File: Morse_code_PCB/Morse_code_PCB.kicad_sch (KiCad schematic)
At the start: 14 parts, among them J1 USB_C_Receptacle_USB2.0, J2 AudioJack3_Ground, J3 AudioJack3_Ground, SW1 RotaryEncoder_Switch, U1 STM32F030F4Px, U2 OLED_12864

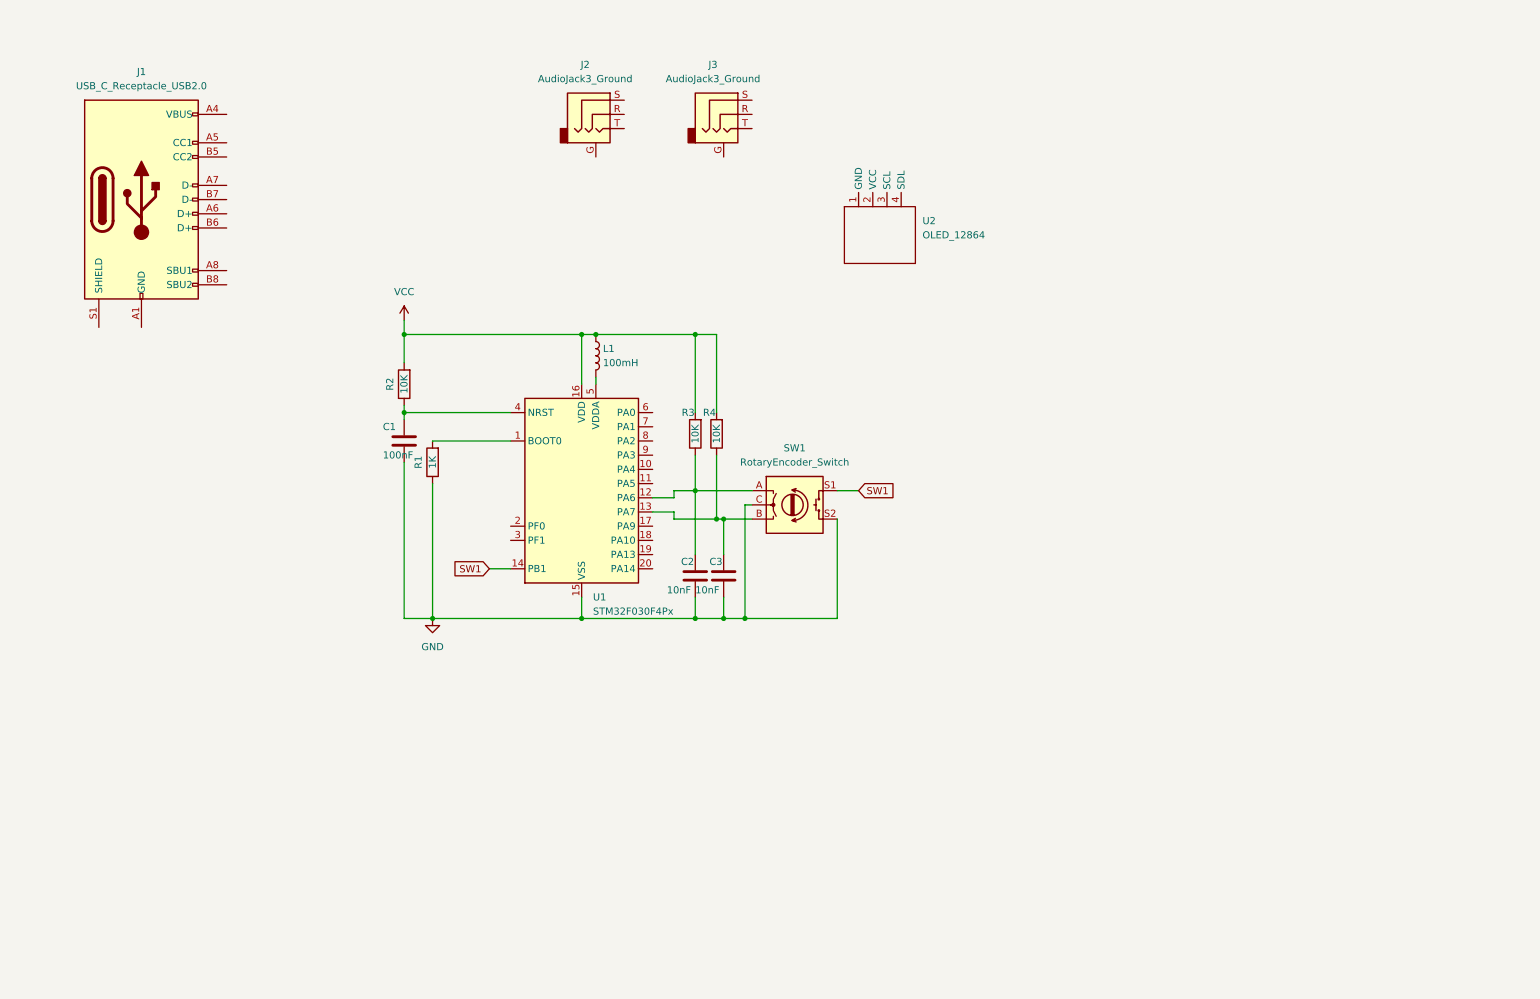
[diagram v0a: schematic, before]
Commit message: 摸鱼画了一点 Signed-off-by: kevin <kevin@lmve.net>
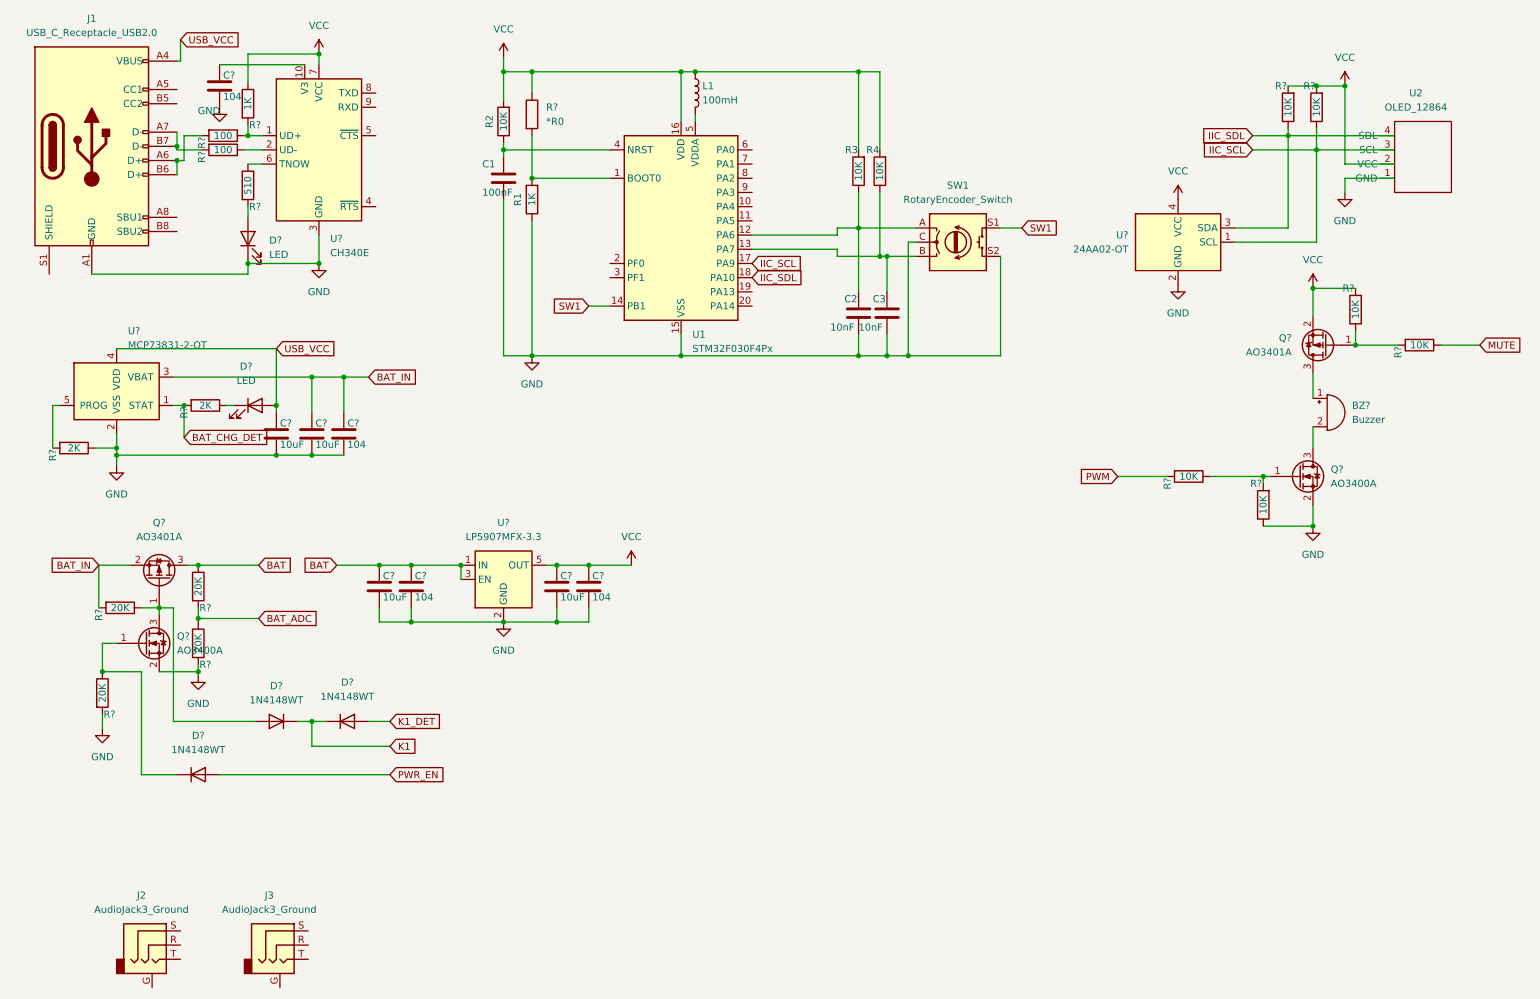
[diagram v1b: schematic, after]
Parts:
- added BZ?: Buzzer, Buzzer_Beeper:Buzzer_TDK_PS1240P02BT_D12.2mm_H6.5mm, symbol Device:Buzzer
- added C? (x4): 10uF, Capacitor_SMD:C_2220_5650Metric, symbol Device:C
- added C? (x4): 104, Capacitor_SMD:C_0805_2012Metric, symbol Device:C
- added D? (x3): 1N4148WT, Diode_SMD:D_SOD-523, symbol Diode:1N4148WT
- added D? (x2): LED, LED_SMD:LED_0603_1608Metric, symbol Device:LED
- added Q? (x2): AO3401A, Package_TO_SOT_SMD:SOT-23, symbol Transistor_FET:AO3401A
- added Q? (x2): AO3400A, Package_TO_SOT_SMD:SOT-23, symbol Transistor_FET:AO3400A
- added R? (x2): 100, Resistor_SMD:R_0603_1608Metric, symbol Device:R
- added R? (x6): 10K, Resistor_SMD:R_0603_1608Metric, symbol Device:R
- added R? (x4): 20K, Resistor_SMD:R_0603_1608Metric, symbol Device:R
- added R?: 510, Resistor_SMD:R_0603_1608Metric, symbol Device:R
- added R? (x2): 2K, Resistor_SMD:R_0603_1608Metric, symbol Device:R
- added R?: 1K, Resistor_SMD:R_0603_1608Metric, symbol Device:R
- added R?: *R0, Resistor_SMD:R_0402_1005Metric, symbol Device:R
- added U?: MCP73831-2-OT, Package_TO_SOT_SMD:SOT-23-5, symbol Battery_Management:MCP73831-2-OT
- added U?: 24AA02-OT, Package_SO:TSSOP-8_4.4x3mm_P0.65mm, symbol Memory_EEPROM:24AA02-OT
- added U?: CH340E, Package_SO:MSOP-10_3x3mm_P0.5mm, symbol Interface_USB:CH340E
- added U?: LP5907MFX-3.3, Package_TO_SOT_SMD:SOT-23-5, symbol Regulator_Linear:LP5907MFX-3.3
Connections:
- net GND: now also J1.A1 (GND), J1.A12 (GND), J1.B1 (GND), J1.B12 (GND), U2.1 (GND), C?.2, C?.2, C?.2, C?.2, C?.2, C?.2, C?.2, C?.2, D?.1 (K), Q?.2 (S), Q?.2 (S), R?.1, R?.1, R?.2, R?.2, U?.2 (GND), U?.2 (GND), U?.2 (VSS), U?.3 (GND)
- net VCC: now also U2.2 (VCC), C?.1, C?.1, Q?.2 (S), R?.1, R?.1, R?.2, R?.2, R?.2, U?.4 (VCC), U?.5 (OUT), U?.7 (VCC)
- net IIC_SCL: now reaches U2.3 (SCL)
- net IIC_SCL: now also U1.17 (PA9), R?.1, U?.1 (SCL)
- net IIC_SDL: now reaches U2.4 (SDL)
- net IIC_SDL: now also U1.18 (PA10), R?.1, U?.3 (SDA)
- net at R1.2, U1.1 (BOOT0): now also R?.2
- net USB_VCC: now reaches J1.A4 (VBUS), J1.A9 (VBUS), J1.B4 (VBUS), J1.B9 (VBUS)
- net USB_VCC: now also C?.1, D?.2 (A), U?.4 (VDD)
- net at J1.A6 (D+): now also J1.B6 (D+), R?.2
- net at J1.A7 (D-): now also J1.B7 (D-), R?.2
- new net: R?.1, R?.2, U?.1 (UD+)
- new net: Q?.1 (G), R?.1, R?.2 (x2)
- new net: D?.2 (A), Q?.1 (G), Q?.3 (D), R?.1
- new net: D?.1 (K), Q?.1 (G), R?.1
- new net: R?.1, U?.2 (UD-)
- new net: R?.1, U?.6 (TNOW)
- new net: D?.2 (A), R?.2
- new net: C?.1, U?.10 (V3)
- new net: BZ?.1 (-), Q?.3 (D)
- new net: BZ?.2 (+), Q?.3 (D)
- new net: D?.1 (K), R?.1
- new net: R?.2, U?.5 (PROG)
- new net BAT: C?.1, C?.1, Q?.3 (D), R?.1, U?.1 (IN), U?.3 (EN)
- new net BAT_ADC: R?.1, R?.2
- new net BAT_CHG_DET: R?.2, U?.1 (STAT)
- new net BAT_IN: C?.1, C?.1, Q?.2 (S), R?.2, U?.3 (VBAT)
- new net K1: D?.1 (K), D?.1 (K)
- new net K1_DET: D?.2 (A)
- new net MUTE: R?.1
- new net PWM: R?.2
- new net PWR_EN: D?.2 (A)
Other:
- moved on the sheet: C1, C2, C3, J1, J2, J3, L1, R1, R2, R3, R4, SW1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
